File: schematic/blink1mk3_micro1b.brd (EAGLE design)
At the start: 88.5 x 50.8 mm, 37 parts, among them J1 NONPOP, U2 EFM32HG309F64G, X2 USBPCB2

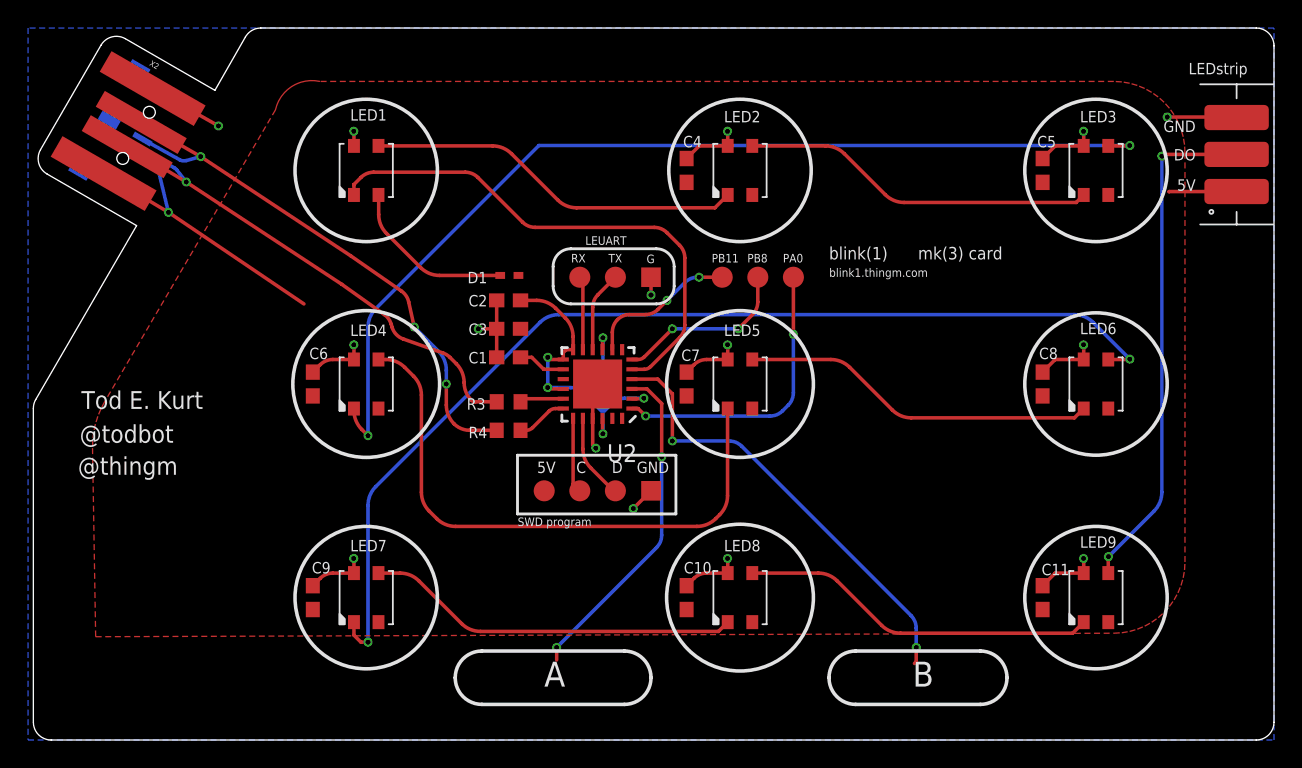
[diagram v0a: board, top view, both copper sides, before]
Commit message: add more micro ideas
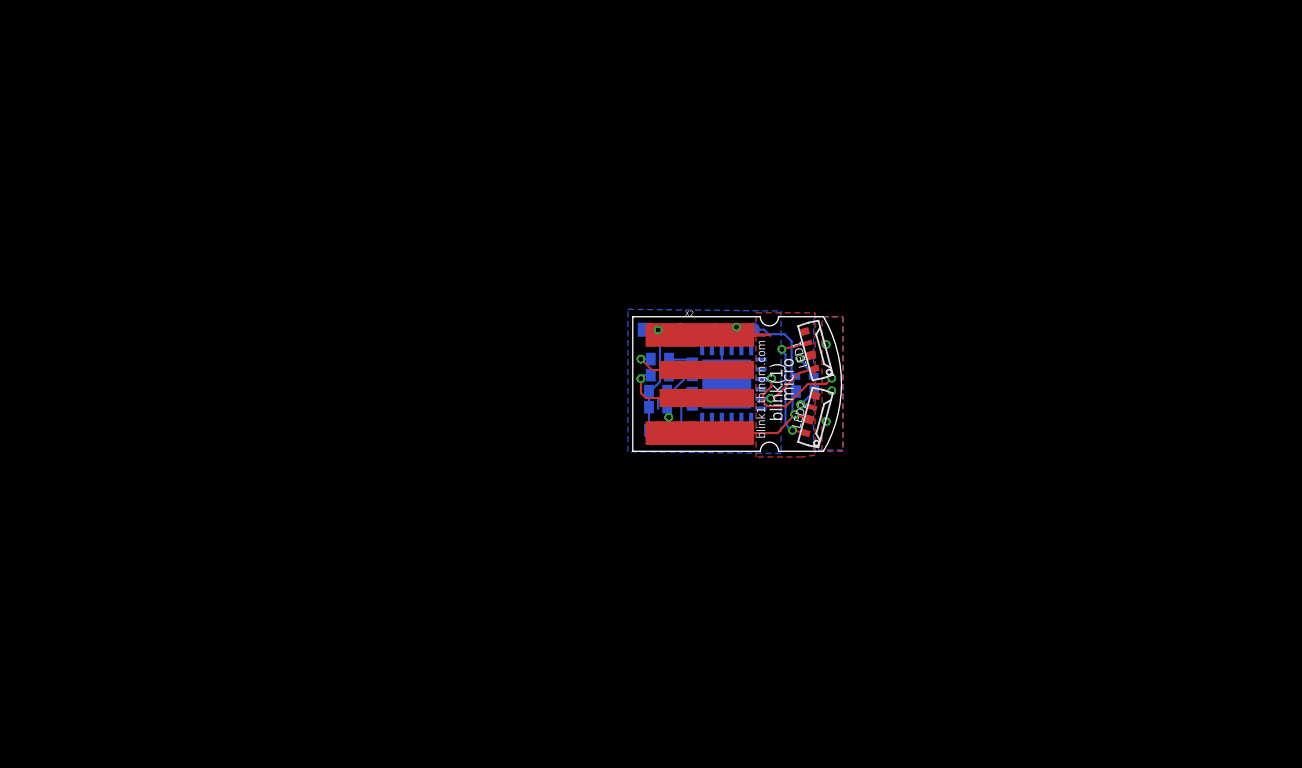
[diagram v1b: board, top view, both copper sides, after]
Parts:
- removed C10, C11, C5, C6, C7, C8, C9: 0.1uF, adafruit:C0603
- removed GND: TPTP14SQ, testpad:TP14SQ
- removed J1: NONPOP, SparkFun-Connectors:USB-B-MICRO-SMD
- removed LED3, LED4, LED5, LED6, LED7, LED8, LED9: SK6812MINI, adafruit:LED3535
- removed PA0, PB11, PB8, RX, TX: TPTP15R, testpad:TP15R
- removed U$1: LED_STRIP_3P, NeoJoints:LEDSTRIP-3P
- removed U2: EFM32HG309F64G, todstuff:QFN24PAD
- added U1: EFM32HG309F64G, todstuff:QFN24PAD
- 5V, C, D: value TPTP15R -> TPTP10R; device testpad:TP15R -> testpad:TP10R
- C1, C2, C3, C4: device adafruit:C0603 -> adafruit:C0402
- G: value TPTP14SQ -> TPTP10SQ; device testpad:TP14SQ -> testpad:TP10SQ
- LED1, LED2: value SK6812MINI -> WS2812B4020SIDE; device adafruit:LED3535 -> todstuff:SK6812-SIDE
- R3, R4: device adafruit:R0603 -> adafruit:R0402
- moved X2 44.5 mm to (4.95, 0.00), turned to 0 degrees
- moved LED1 34.6 mm to (11.8, 2.40), turned to 285 degrees
- moved D1 22.4 mm to (11.0, 0.55), flipped to the bottom
- moved 5V 18.8 mm to (7.29, 3.87), flipped to the bottom
- moved LED2 18.5 mm to (11.8, -2.40), turned to 255 degrees
- moved C4 17.9 mm to (11.0, -0.53), flipped to the bottom, turned to 180 degrees
- moved C 13.6 mm to (2.11, 3.88), flipped to the bottom
- moved D 13.5 mm to (4.59, 3.87), flipped to the bottom
- moved C2 12.5 mm to (0.51, -0.51), flipped to the bottom, turned to 0 degrees
- moved C3 12.0 mm to (0.51, -1.65), flipped to the bottom, turned to 0 degrees
- moved R4 11.9 mm to (0.64, 1.78), flipped to the bottom, turned to 0 degrees
- moved C1 11.9 mm to (0.51, -3.30), flipped to the bottom, turned to 0 degrees
- moved R3 11.0 mm to (0.64, 0.64), flipped to the bottom, turned to 0 degrees
- moved G 3.77 mm to (-0.44, 3.87), flipped to the bottom
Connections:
- removed net N$10: LED6.3, LED7.1
- removed net N$4: LED7.3, LED8.1
- removed net N$5: LED4.3, LED5.1
- removed net N$6: LED5.3, LED6.1
- removed net N$7: LED2.3, LED3.1
- removed net N$8: LED3.3, LED4.1
- removed net N$9: LED8.3, LED9.1
- removed net PA0: PA0.TP, U2.1
- removed net PB11: PB11.TP, U2.8
- removed net PB8: PB8.TP, U2.6
- new net LED1: U1.1
- new net N$1: U1.8
- new net N$3: U1.6
- net +3V3: now also U1.12, U1.13, U1.16, U1.2, U1.22, U1.9; no longer U2.12, U2.13, U2.16, U2.2, U2.22, U2.9
- net +5V: now also LED2.1-VDD, U1.15; no longer C10.1, C11.1, C5.1, C6.1, C7.1, C8.1, C9.1, J1.VBUS, LED2.2, LED3.2, LED4.2, LED5.2, LED6.2, LED7.2, LED8.2, LED9.2, U$1.A, U2.15
- net /RESET: now also U1.7; no longer U2.7
- net CAP0A: now also U1.3; no longer U2.3
- net CAP0B: now also U1.23; no longer U2.23
- net CAP1A: now also U1.4; no longer U2.4
- net CAP1B: now also U1.24; no longer U2.24
- net DBG_SWCLK: now also U1.19; no longer U2.19
- net DBG_SWDIO: now also U1.20; no longer U2.20
- net DECOUPLE: now also U1.14; no longer U2.14
- net DI: now also LED1.4-DIN, U1.5; no longer LED1.1, U2.5
- net DO: now also LED2.2-DOUT; no longer LED9.3, U$1.B
- net GND: now also LED1.3-GND, LED2.3-GND, U1.21, U1.PAD; no longer C10.2, C11.2, C5.2, C6.2, C7.2, C8.2, C9.2, GND.TP, J1.GND, LED1.4, LED2.4, LED3.4, LED4.4, LED5.4, LED6.4, LED7.4, LED8.4, LED9.4, U$1.C, U2.21, U2.PAD
- net LEUO_RX: now also U1.11; no longer RX.TP, U2.11
- net LEUO_TX: now also U1.10; no longer TX.TP, U2.10
- net N$2: now also LED1.2-DOUT, LED2.4-DIN; no longer LED1.3, LED2.1
- net RUSB_D+: now also U1.18; no longer U2.18
- net RUSB_D-: now also U1.17; no longer U2.17
- net USB_D+: no longer J1.D+
- net USB_D-: no longer J1.D-
- net VLEDA: now also LED1.1-VDD; no longer LED1.2
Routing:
- net N$10: track 74.9 -> 0.00 mm, vias 2 -> 0
- net N$8: track 71.7 -> 0.00 mm, vias 2 -> 0
- net N$5: track 41.7 -> 0.00 mm
- net DO: track 36.6 -> 0.00 mm, vias 2 -> 0
- net USB_D+: track 40.5 -> 5.73 mm, vias 3 -> 1
- net GND: track 59.2 -> 26.1 mm, vias 15 -> 3
- net DI: track 37.2 -> 4.71 mm, vias 0 -> 1
- net CAP1A: track 32.3 -> 0.00 mm, vias 2 -> 0
- net USB_D-: track 37.3 -> 6.68 mm
- net N$4: track 26.7 -> 0.00 mm
- net +3V3: track 29.3 -> 3.12 mm, vias 5 -> 0
- net N$9: track 25.5 -> 0.00 mm
- net N$6: track 25.4 -> 0.00 mm
- net N$7: track 25.3 -> 0.00 mm
- net PA0: track 20.8 -> 0.00 mm, vias 2 -> 0
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- added copper zone on layer 16, net +3V3
- added copper zone on layer 16, net CAP0A
- added copper zone on layer 1, net GND
- removed copper zone on layer 1, net +5V
- removed copper zone on layer 1, net CAP1A
- removed copper zone on layer 16, net GND
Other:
- board size 88.5 x 50.8 mm -> 14.9 x 9.6 mm
- board text added: "blink1mk3micro1a"
- board text added: "micro"
- board text removed: "5V"
- board text removed: "@thingm"
- board text removed: "@todbot"
- board text removed: "A"
- board text removed: "B"
- board text removed: "DO"
- board text removed: "GND"
- board text removed: "Gnd"
- board text removed: "LEDstrip"
- board text removed: "LEUART"
- board text removed: "SWD program"
- board text removed: "Tod E. Kurt"
- board text removed: "blink1mk3_card"
- board text removed: "mk(3) card"
